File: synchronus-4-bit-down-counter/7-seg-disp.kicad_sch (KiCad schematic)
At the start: 22 parts, among them SW3 data, U10 HDSP-5553-7-segment-cc, U11 4071-quad-OR, U12 4071-quad-OR, U13 4071-quad-OR, U14 4071-quad-OR, U15 4081-quad-AND, U16 4081-quad-AND, U17 4081-quad-AND, U7 4069, U9 4071-quad-OR

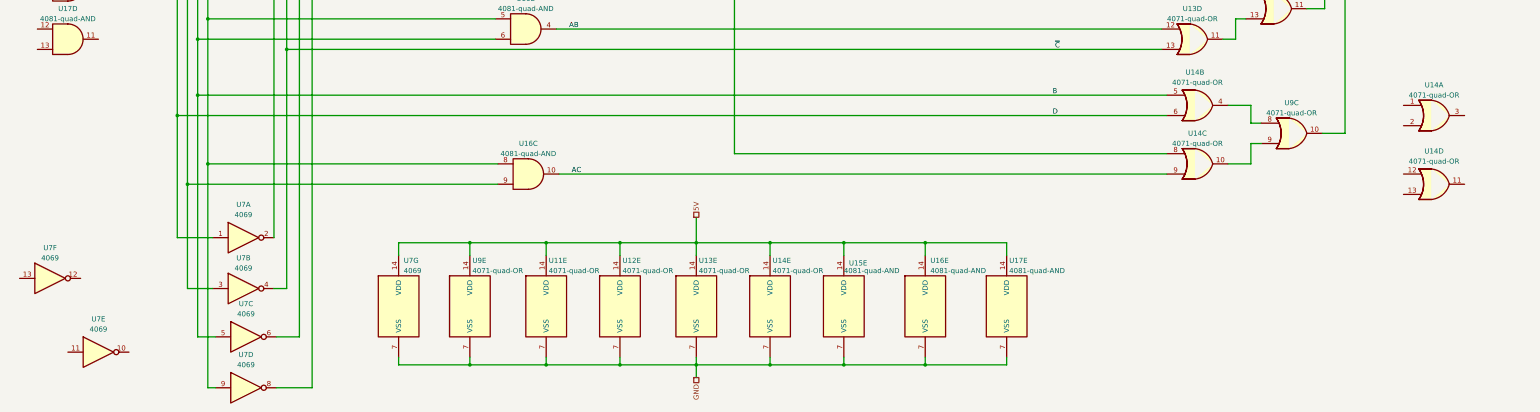
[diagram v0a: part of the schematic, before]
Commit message: sdvsdv
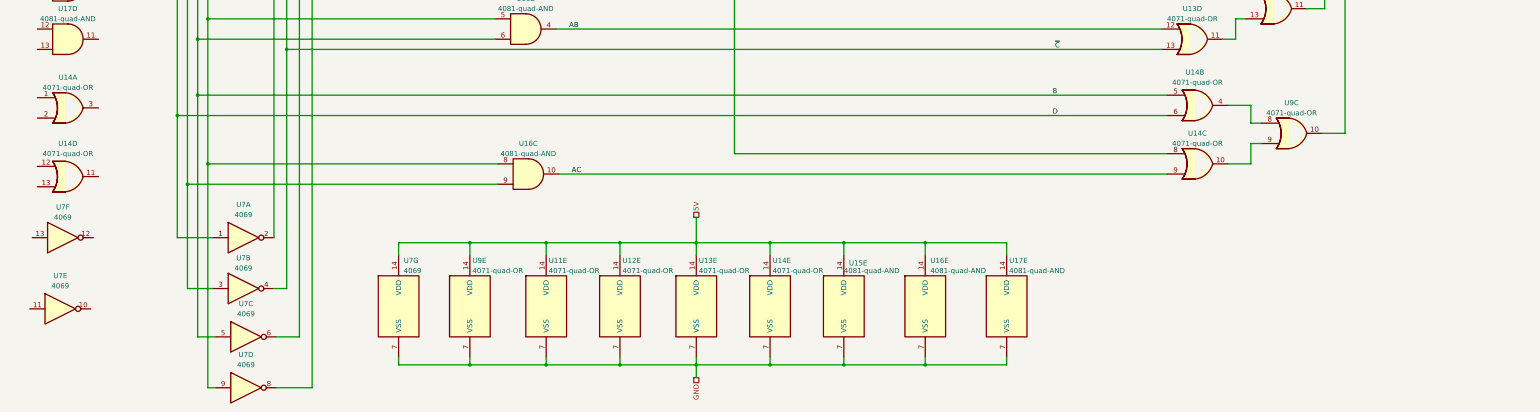
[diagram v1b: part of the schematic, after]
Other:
- moved on the sheet: U14A, U14D, U7E, U7F
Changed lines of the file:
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@@
     )
   )
-  (symbol (lib_id "000_Logic_IC_Immo:4071-quad-OR") (at 368.3 212.09 0) (unit 1)
-    (in_bom yes) (on_board yes) (dnp no) (fields_autoplaced)
-    (property "Reference" "U14" (at 368.3 204.47 0)
-      (effects (font (size 1.27 1.27)))
-    )
-    (property "Value" "4071-quad-OR" (at 368.3 207.01 0)
-      (effects (font (size 1.27 1.27)))
-    )
-    (property "Footprint" "" (at 368.3 212.09 0)
-      (effects (font (size 1.27 1.27)) hide)
-    )
-    (property "Datasheet" "http://www.intersil.com/content/dam/Intersil/documents/cd40/cd4071bms-72bms-75bms.pdf" (at 368.3 212.09 0)
+  (symbol (lib_id "000_Logic_IC_Immo:4071-quad-OR") (at 27.305 210.185 0) (unit 1)
+    (in_bom yes) (on_board yes) (dnp no) (fields_autoplaced)
+    (property "Reference" "U14" (at 27.305 202.565 0)
+      (effects (font (size 1.27 1.27)))
+    )
+    (property "Value" "4071-quad-OR" (at 27.305 205.105 0)
+      (effects (font (size 1.27 1.27)))
+    )
+    (property "Footprint" "" (at 27.305 210.185 0)
+      (effects (font (size 1.27 1.27)) hide)
+    )
+    (property "Datasheet" "http://www.intersil.com/content/dam/Intersil/documents/cd40/cd4071bms-72bms-75bms.pdf" (at 27.305 210.185 0)
       (effects (font (size 1.27 1.27)) hide)
     )
@@
     )
   )
-  (symbol (lib_id "000_Logic_IC_Immo:4071-quad-OR") (at 368.3 229.235 0) (unit 4)
-    (in_bom yes) (on_board yes) (dnp no) (fields_autoplaced)
-    (property "Reference" "U14" (at 368.3 220.98 0)
-      (effects (font (size 1.27 1.27)))
-    )
-    (property "Value" "4071-quad-OR" (at 368.3 223.52 0)
-      (effects (font (size 1.27 1.27)))
-    )
-    (property "Footprint" "" (at 368.3 229.235 0)
-      (effects (font (size 1.27 1.27)) hide)
-    )
-    (property "Datasheet" "http://www.intersil.com/content/dam/Intersil/documents/cd40/cd4071bms-72bms-75bms.pdf" (at 368.3 229.235 0)
+  (symbol (lib_id "000_Logic_IC_Immo:4071-quad-OR") (at 27.305 227.33 0) (unit 4)
+    (in_bom yes) (on_board yes) (dnp no) (fields_autoplaced)
+    (property "Reference" "U14" (at 27.305 219.075 0)
+      (effects (font (size 1.27 1.27)))
+    )
+    (property "Value" "4071-quad-OR" (at 27.305 221.615 0)
+      (effects (font (size 1.27 1.27)))
+    )
+    (property "Footprint" "" (at 27.305 227.33 0)
+      (effects (font (size 1.27 1.27)) hide)
+    )
+    (property "Datasheet" "http://www.intersil.com/content/dam/Intersil/documents/cd40/cd4071bms-72bms-75bms.pdf" (at 27.305 227.33 0)
       (effects (font (size 1.27 1.27)) hide)
     )
@@
     )
   )
-  (symbol (lib_id "4xxx:4069") (at 34.925 271.145 0) (unit 5)
-    (in_bom yes) (on_board yes) (dnp no) (fields_autoplaced)
-    (property "Reference" "U7" (at 34.925 262.89 0)
-      (effects (font (size 1.27 1.27)))
-    )
-    (property "Value" "4069" (at 34.925 265.43 0)
-      (effects (font (size 1.27 1.27)))
-    )
-    (property "Footprint" "" (at 34.925 271.145 0)
-      (effects (font (size 1.27 1.27)) hide)
-    )
-    (property "Datasheet" "http://www.intersil.com/content/dam/Intersil/documents/cd40/cd4069ubms.pdf" (at 34.925 271.145 0)
+  (symbol (lib_id "4xxx:4069") (at 25.4 260.35 0) (unit 5)
+    (in_bom yes) (on_board yes) (dnp no) (fields_autoplaced)
+    (property "Reference" "U7" (at 25.4 252.095 0)
+      (effects (font (size 1.27 1.27)))
+    )
+    (property "Value" "4069" (at 25.4 254.635 0)
+      (effects (font (size 1.27 1.27)))
+    )
+    (property "Footprint" "" (at 25.4 260.35 0)
+      (effects (font (size 1.27 1.27)) hide)
+    )
+    (property "Datasheet" "http://www.intersil.com/content/dam/Intersil/documents/cd40/cd4069ubms.pdf" (at 25.4 260.35 0)
       (effects (font (size 1.27 1.27)) hide)
     )
@@
     )
   )
-  (symbol (lib_id "4xxx:4069") (at 22.86 252.73 0) (unit 6)
-    (in_bom yes) (on_board yes) (dnp no) (fields_autoplaced)
-    (property "Reference" "U7" (at 22.86 245.11 0)
-      (effects (font (size 1.27 1.27)))
-    )
-    (property "Value" "4069" (at 22.86 247.65 0)
-      (effects (font (size 1.27 1.27)))
-    )
-    (property "Footprint" "" (at 22.86 252.73 0)
-      (effects (font (size 1.27 1.27)) hide)
-    )
-    (property "Datasheet" "http://www.intersil.com/content/dam/Intersil/documents/cd40/cd4069ubms.pdf" (at 22.86 252.73 0)
-      (effects (font (size 1.27 1.27)) hide)
-    )
+  (symbol (lib_id "4xxx:4069") (at 26.035 242.57 0) (unit 6)
+    (in_bom yes) (on_board yes) (dnp no) (fields_autoplaced)
+    (property "Reference" "U7" (at 26.035 234.95 0)
+      (effects (font (size 1.27 1.27)))
+    )
+    (property "Value" "4069" (at 26.035 237.49 0)
+      (effects (font (size 1.27 1.27)))
+    )
+    (property "Footprint" "" (at 26.035 242.57 0)
+      (effects (font (size 1.27 1.27)) hide)
+    )
+    (property "Datasheet" "http://www.intersil.com/content/dam/Intersil/documents/cd40/cd4069ubms.pdf" (at 26.035 242.57 0)
+      (effects (font (size 1.27 1.27)) hide)
+    )
